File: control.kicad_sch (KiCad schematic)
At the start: 9 parts, among them U201 ICE40HX8K-BG121, U202 TMUX1104, U203 SLG46621

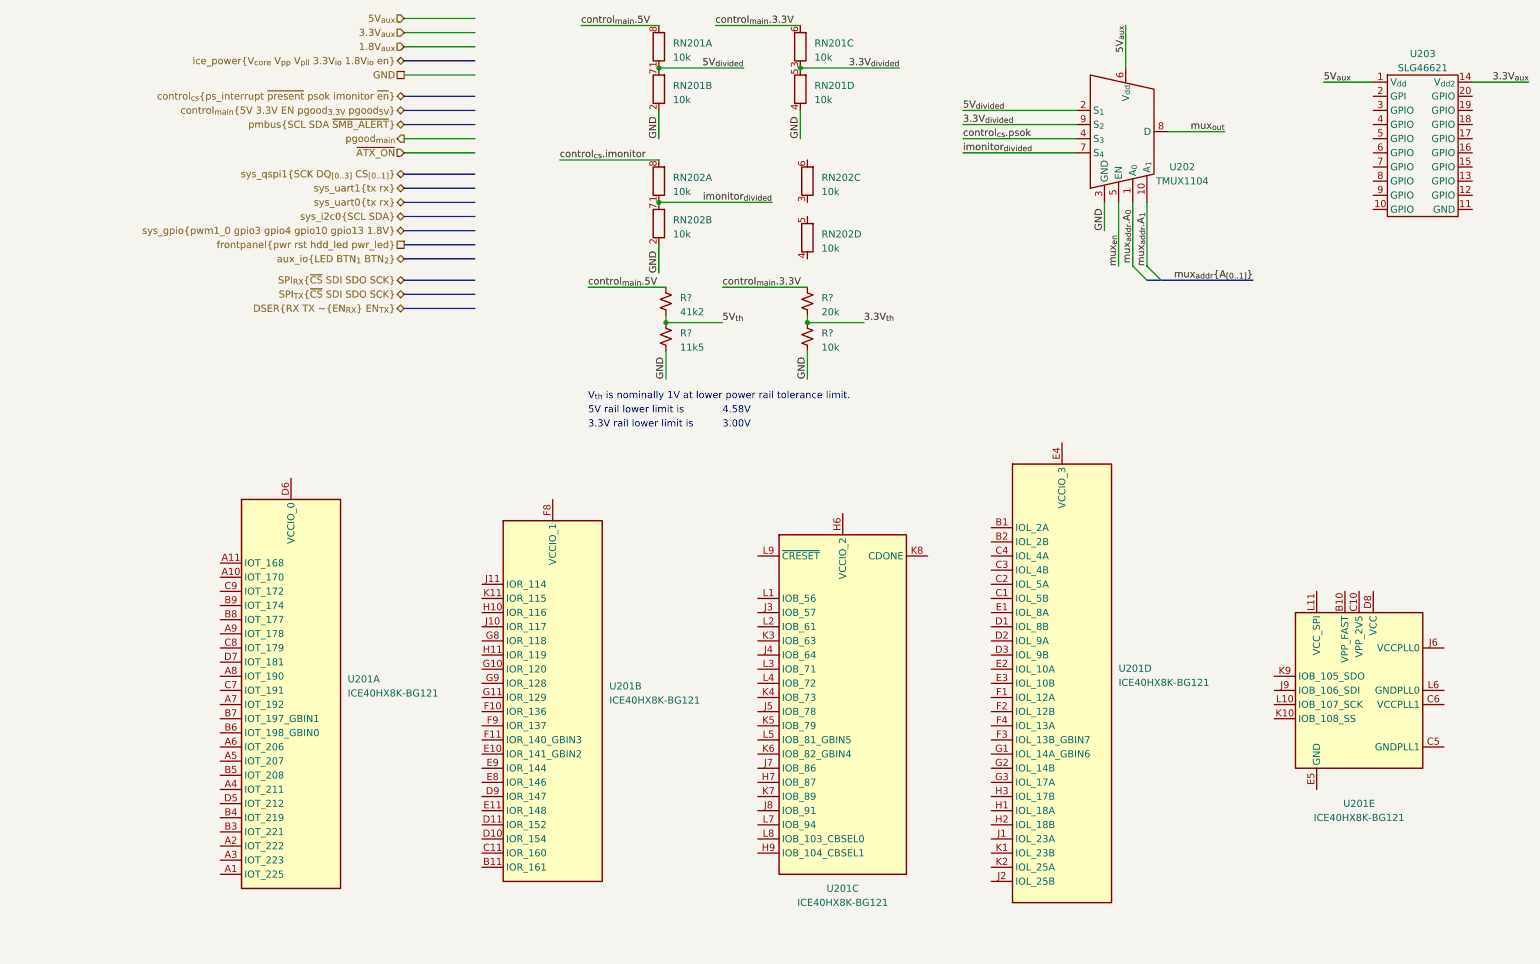
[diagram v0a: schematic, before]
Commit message: tweak schematic
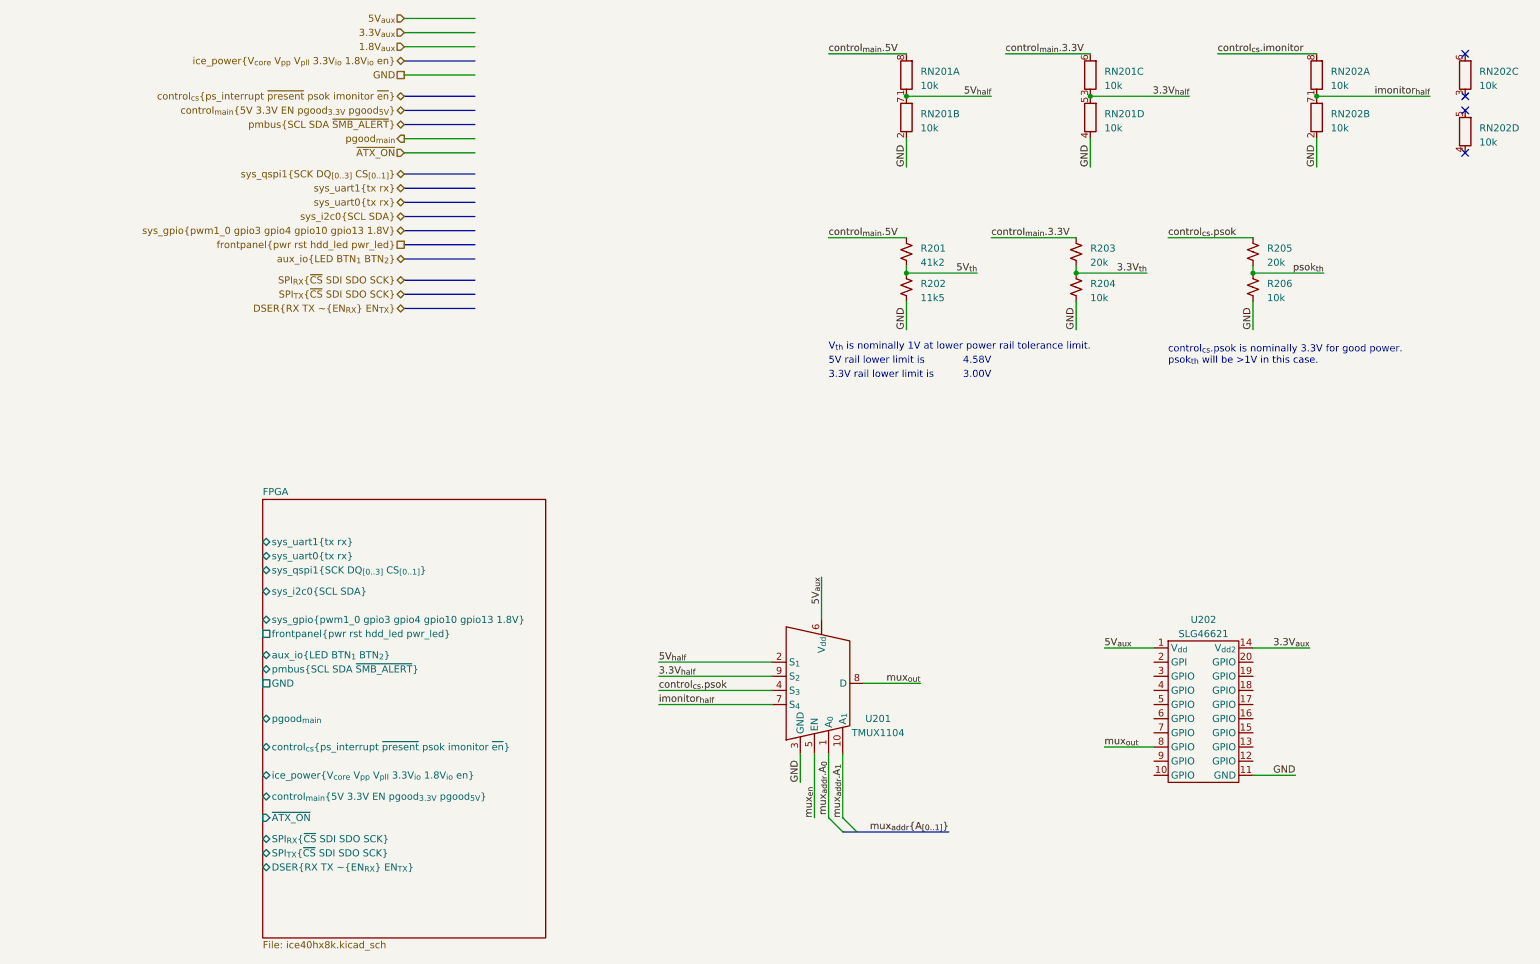
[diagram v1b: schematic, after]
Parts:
- removed U201: ICE40HX8K-BG121, Package_BGA:BGA-121_9.0x9.0mm_Layout11x11_P0.8mm_Ball0.4mm_Pad0.35mm_NSMD, symbol proj_sym:ICE40HX8K-BG121
- added R205: 20k, symbol proj_sym:Resistor
- added R206: 10k, symbol proj_sym:Resistor
- gave numbers to parts that had none: 4
- renumbered U202 to U201, U203 to U202
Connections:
- net GND: now also U202.11 (GND), R206.2
- net control_{cs}.psok: now also R205.1
- net mux_{out}: now also U202.8 (GPIO)
- net 3.3V_{divided} renamed 3.3V_{half}
- net 5V_{divided} renamed 5V_{half}
- net imonitor_{divided} renamed imonitor_{half}
- new net psok_{th}: R205.2, R206.1
- no-connect marks 0 -> 4
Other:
- added sheet FPGA (ice40hx8k.kicad_sch)
- note added: "control_{cs}.psok is nominally 3.3V for good power. psok_{th} will be >1V in this case."
- moved on the sheet: R201, R202, R203, R204, RN201A, RN201B, RN201C, RN201D, RN202A, RN202B, RN202C, RN202D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
